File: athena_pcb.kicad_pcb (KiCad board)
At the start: 2 copper layers, 40.5 x 23.8 mm, 36 parts, among them J2 Conn_01x04, SW1 SW_Push, U1 NRF5340-QKAA-R7, U2 BME280, Y1 32MHz, Y2 32.768kHz

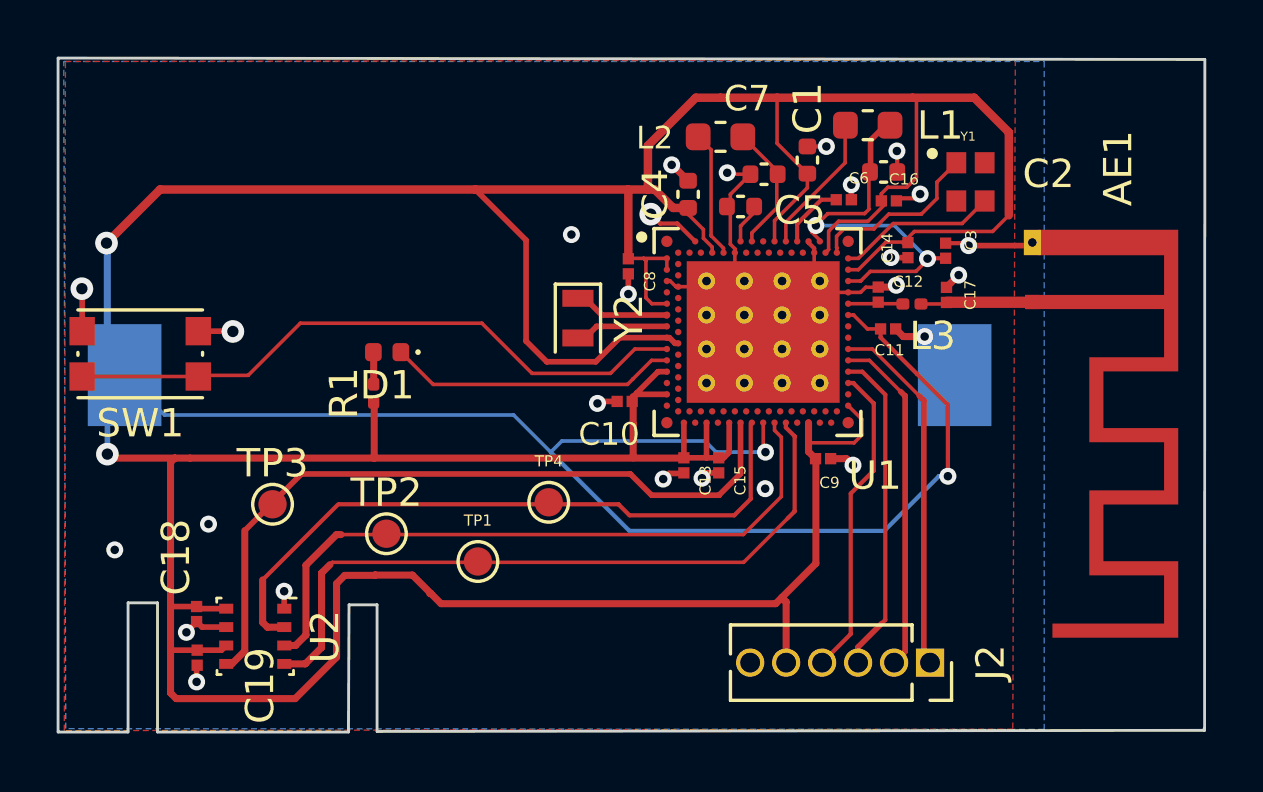
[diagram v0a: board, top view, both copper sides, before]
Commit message: Changes from the review
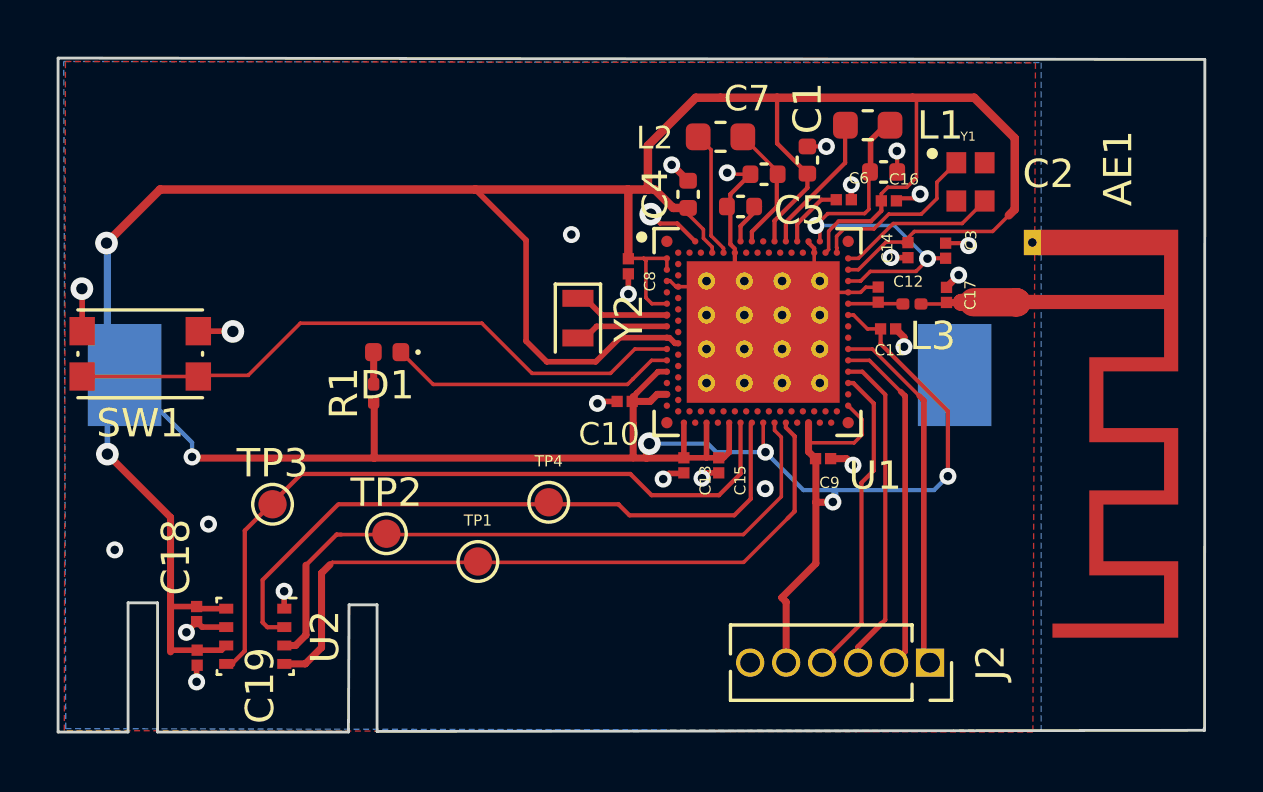
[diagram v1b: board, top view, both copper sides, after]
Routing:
- net VDD: track 218.6 -> 167.2 mm, vias 4 -> 7
- net GND: track 43.3 -> 38.8 mm, vias 26 -> 25
